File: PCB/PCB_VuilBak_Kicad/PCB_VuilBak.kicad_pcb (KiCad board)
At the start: 2 copper layers, 7.6 x 1.2 mm, 39 parts, among them Q1 2N7002, Q2 2N7002, U1 micro_usb, U2 AMS1117-3.3, U3 TCA9548A_I2C_Multiplexer, U4 esp_wroom_32, X1 DG3XX-04-3.5, X10 DG3XX-04-3.5, X11 DG3XX-02-3.5, X12 DG3XX-02-3.5, X13 DG3XX-02-3.5, X2 DG3XX-04-3.5, X3 DG3XX-04-3.5, X4 DG3XX-04-3.5, X5 DG3XX-03-3.5, X6 DG3XX-07-3.5, X7 DG3XX-04-3.5, X8 DG3XX-04-3.5, X9 DG3XX-04-3.5

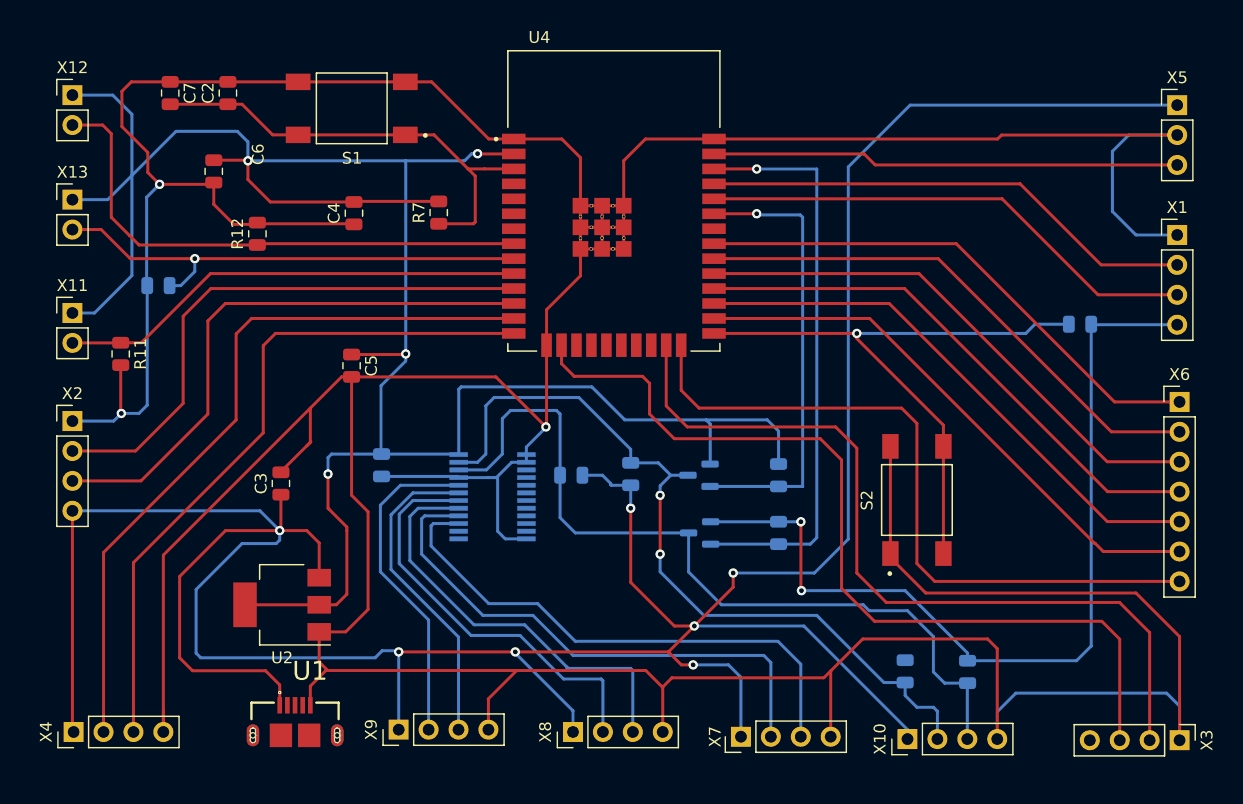
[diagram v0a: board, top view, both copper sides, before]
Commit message: pcb update
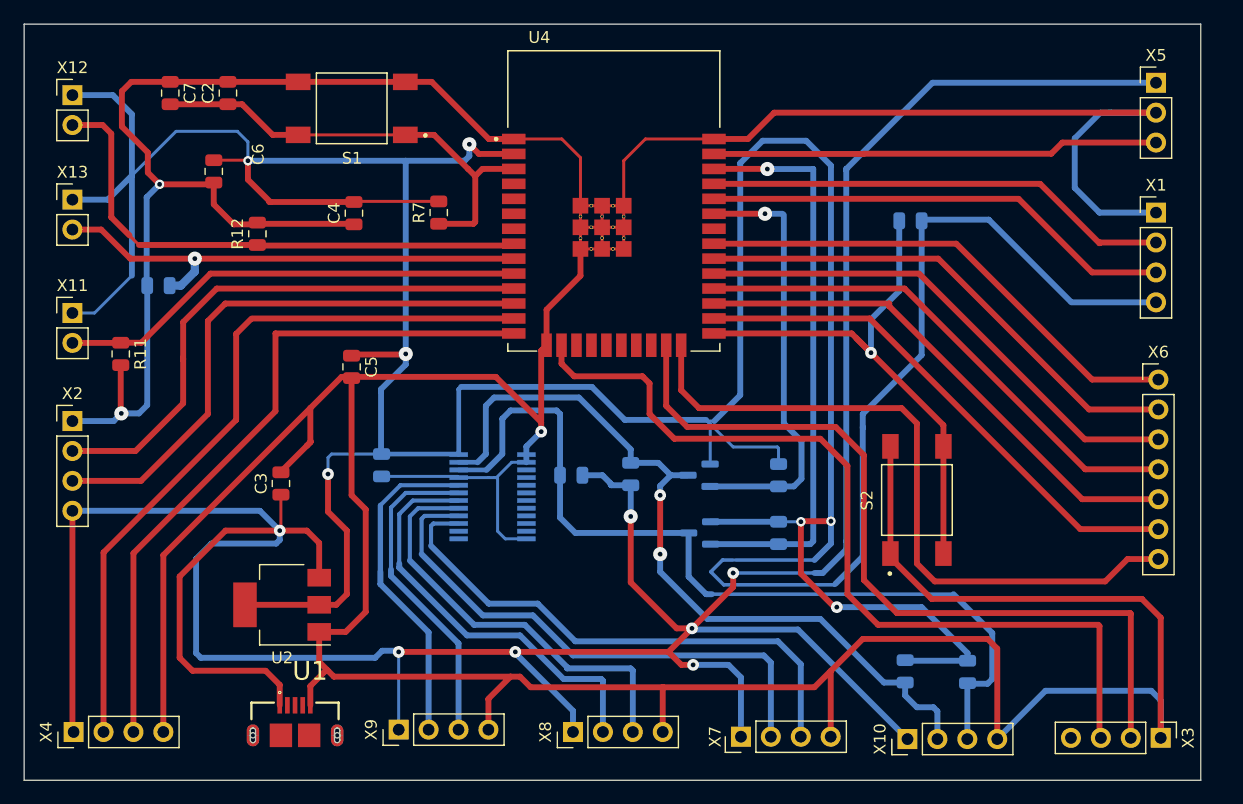
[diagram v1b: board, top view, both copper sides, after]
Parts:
- moved R8 16.9 mm to (172.7, 44.3)
- moved X1 2.62 mm to (193.5, 43.6)
- moved X5 2.62 mm to (193.5, 32.6)
- moved X6 2.62 mm to (193.7, 57.8)
- moved X3 1.61 mm to (193.9, 88.2)
- moved C5 0.10 mm to (125.2, 56.7)
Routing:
- net 3.3V: track 270.0 -> 376.7 mm, vias 6 -> 7
- net SCL_Mux: track 70.3 -> 75.3 mm
- net Net-(R8-Pad1): track 51.8 -> 47.3 mm
- net GND: track 483.3 -> 479.8 mm
- net GPIO4: track 47.7 -> 45.1 mm
- net GPIO 17: track 46.7 -> 44.1 mm
- net GPIO 5: track 46.1 -> 43.6 mm
- net RX: track 42.9 -> 40.3 mm
- net GPIO 19: track 45.1 -> 42.5 mm
- net GPIO 18: track 45.6 -> 43.0 mm
- net TX: track 42.2 -> 39.6 mm
- net GPIO 16: track 47.2 -> 44.7 mm
- net GPIO 23: track 40.1 -> 38.3 mm
- net SDA_ESP: track 38.4 -> 37.0 mm
- net GPIO13: track 75.1 -> 73.9 mm
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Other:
- board size 7.6 x 1.2 mm -> 99.9 x 64.2 mm
